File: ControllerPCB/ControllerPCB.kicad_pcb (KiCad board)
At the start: 4 copper layers, 55 x 90 mm, 43 parts, among them J1 USB_B_Micro, J2 A-DF 09 A/KG-T4S, J3 Screw_Terminal_01x02, J4 MotorDriverSocket, J5 UISocket, J6 Pi JST, J7 Conn_02x02_Row_Letter_First, SW1 SW_Push_Dual_x2, SW2 SW_Push_Dual_x2, U1 AMS1117-3.3, U2 ESP32-S3-WROOM-2, U3 LM1084-5.0, U5 TMP236A4DCKR

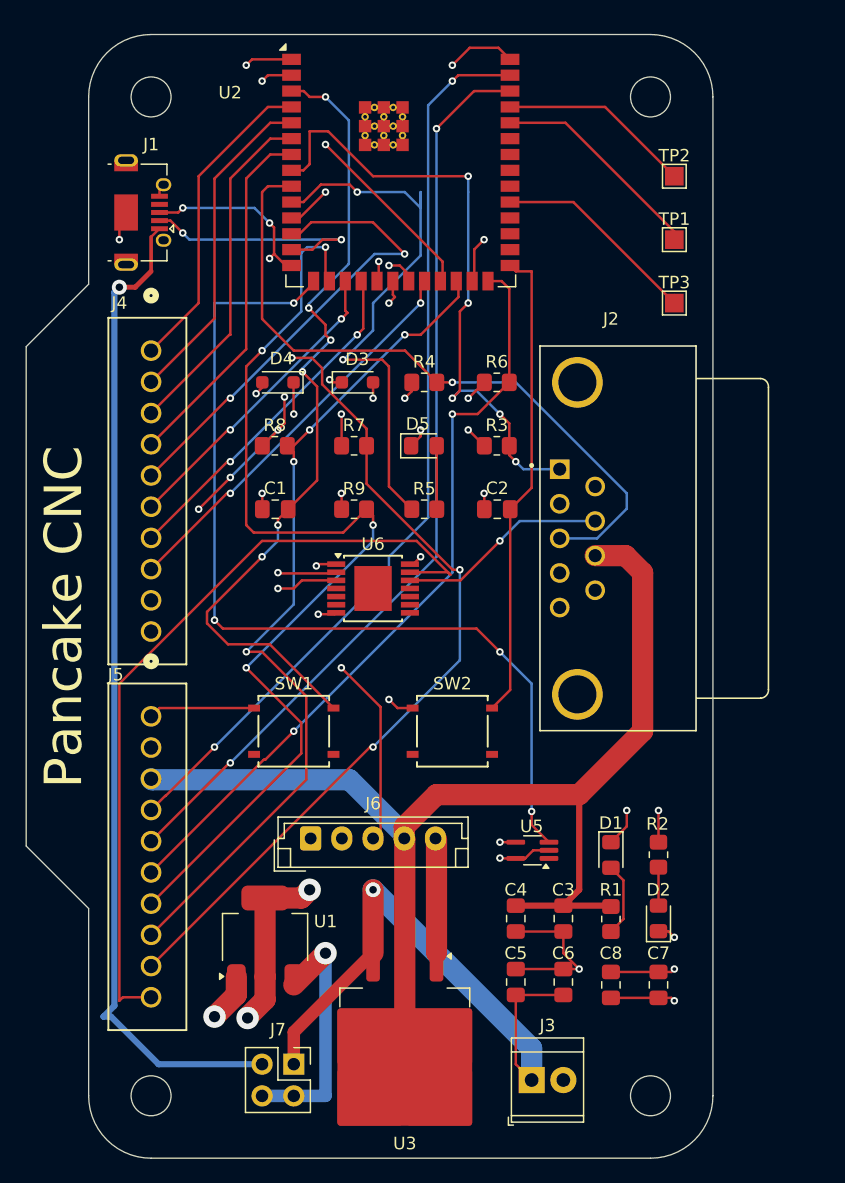
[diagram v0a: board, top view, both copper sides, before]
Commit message: Rev 2 of controller PCB
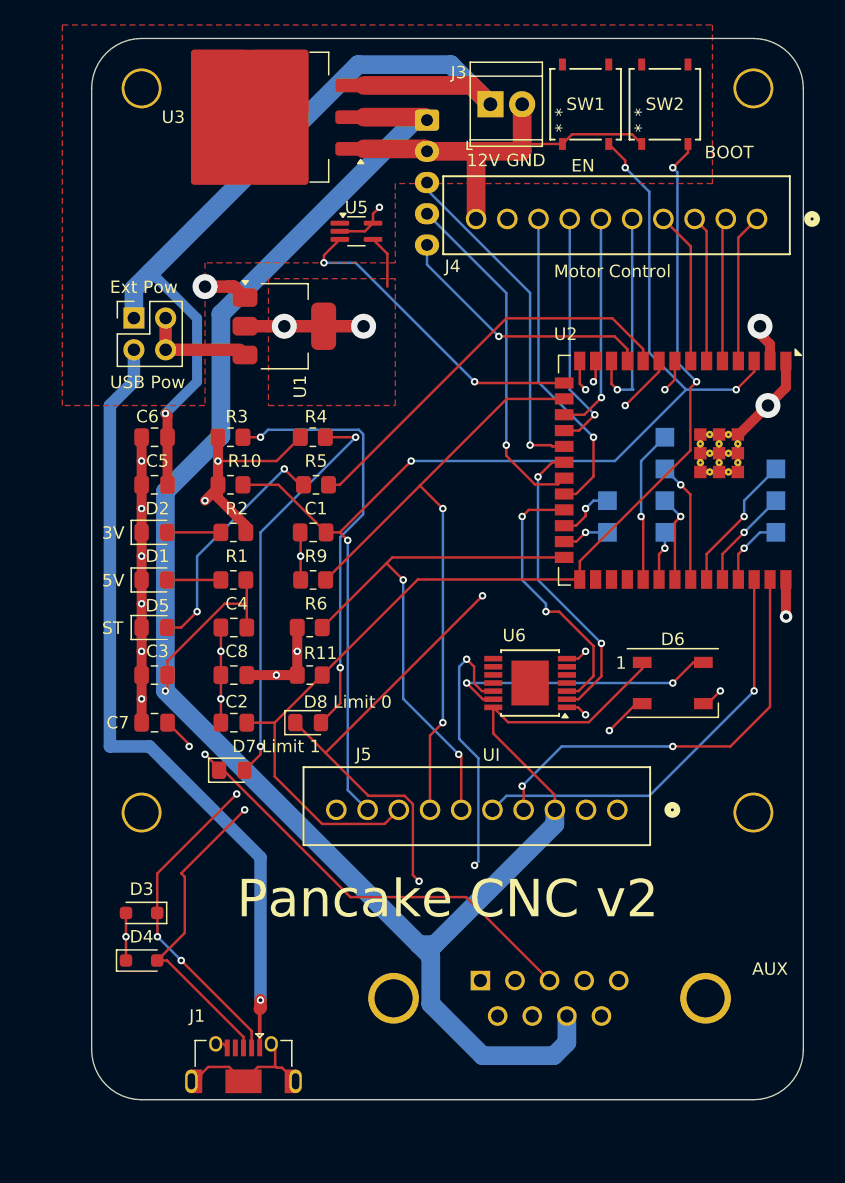
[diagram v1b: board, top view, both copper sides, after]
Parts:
- removed R7, R8: 10k, Resistor_SMD:R_0805_2012Metric_Pad1.20x1.40mm_HandSolder
- added D6: WS2812B, LED_SMD:LED_WS2812B_PLCC4_5.0x5.0mm_P3.2mm, F.Cu at (74.8, 97.9)
- added D7 Limit 1: LED, LED_SMD:LED_0805_2012Metric_Pad1.15x1.40mm_HandSolder, F.Cu at (39.5, 104.9)
- added D8 Limit 0: LED, LED_SMD:LED_0805_2012Metric_Pad1.15x1.40mm_HandSolder, F.Cu at (45.6, 101.1)
- added R10: 10k, Resistor_SMD:R_0805_2012Metric_Pad1.20x1.40mm_HandSolder, F.Cu at (39.4, 82.1)
- added R11: 10k, Resistor_SMD:R_0805_2012Metric_Pad1.20x1.40mm_HandSolder, F.Cu at (45.7, 97.3)
- added TP4: TestPoint, TestPoint:TestPoint_Pad_1.5x1.5mm, B.Cu at (74.2, 85.9)
- added TP5: TestPoint, TestPoint:TestPoint_Pad_1.5x1.5mm, B.Cu at (74.2, 83.3)
- added TP6: TestPoint, TestPoint:TestPoint_Pad_1.5x1.5mm, B.Cu at (74.2, 80.8)
- added TP7: TestPoint, TestPoint:TestPoint_Pad_1.5x1.5mm, B.Cu at (83.0, 80.8)
- added TP8: TestPoint, TestPoint:TestPoint_Pad_1.5x1.5mm, B.Cu at (69.6, 83.3)
- added TP9: TestPoint, TestPoint:TestPoint_Pad_1.5x1.5mm, B.Cu at (69.6, 85.9)
- J2, J6, TP1, TP2, TP3: moved to B.Cu
- R3, R4: value 10k -> 5.1k
- moved J3 78.2 mm to (60.2, 51.6)
- moved U3 75.4 mm to (42.4, 52.6), turned to 180 degrees
- moved J1 70.2 mm to (40.4, 129.8), turned to 0 degrees
- moved J7 61.1 mm to (31.6, 68.7), turned to 90 degrees
- moved J6 58.3 mm to (55.1, 52.9), turned to -90 degrees
- moved SW1 55.4 mm to (67.8, 51.6), turned to 90 degrees
- moved C6 54.5 mm to (33.3, 78.3), turned to 180 degrees
- moved SW2 53.0 mm to (74.2, 51.6), turned to 90 degrees
- moved U5 51.5 mm to (49.4, 61.8), turned to 0 degrees
- moved D2 50.9 mm to (33.3, 85.9), turned to 0 degrees
- moved J4 49.7 mm to (81.5, 60.8), turned to 180 degrees
- moved C5 49.2 mm to (33.3, 82.1), turned to 180 degrees
- moved U1 49.0 mm to (43.7, 69.4), turned to 0 degrees
- moved D4 47.6 mm to (32.2, 120.2), turned to 0 degrees
- moved D3 45.9 mm to (32.2, 116.4), turned to 180 degrees
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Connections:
- C1 pad 2: Net-(SW1A-D) -> Net-(J5-Pin_9)
- C2 pad 2: Net-(SW2A-D) -> Net-(J5-Pin_8)
- J2 pad 1: Net-(U2-IO15) -> Net-(D8-K)
- J2 pad 3: Net-(U2-IO16) -> Net-(D7-K)
- J5 pad 10: Net-(J5-Pin_10) -> Net-(D6-DOUT)
- J6 pad 1: Net-(J6-Pin_1) -> +5V
- J6 pad 2: Net-(J6-Pin_2) -> GND
- J6 pad 4: +5V -> Net-(J6-Pin_4)
- J6 pad 5: GND -> Net-(J6-Pin_5)
- R3 pad 2: Net-(U2-IO15) -> Net-(D8-A)
- R4 pad 2: Net-(U2-IO16) -> Net-(D7-A)
- SW1 pad 2: Net-(SW1A-D) -> (no net)
- SW1 pad 3: (no net) -> Net-(J5-Pin_9)
- SW2 pad 2: Net-(SW2A-D) -> (no net)
- SW2 pad 3: (no net) -> Net-(J5-Pin_8)
- U2 pad 11: Net-(J6-Pin_3) -> Net-(J6-Pin_5)
- U2 pad 19: Net-(J6-Pin_1) -> Net-(J6-Pin_3)
- U2 pad 21: Net-(J6-Pin_2) -> Net-(J6-Pin_4)
- U2 pad 24: Net-(J5-Pin_8) -> Net-(U2-IO47)
- U2 pad 25: Net-(J5-Pin_9) -> Net-(U2-IO48)
- U2 pad 27: Net-(SW2A-D) -> Net-(J5-Pin_8)
- U2 pad 3: Net-(SW1A-D) -> Net-(J5-Pin_9)
- U2 pad 32: unconnected-(U2-MTCK/IO39-Pad32) -> Net-(U2-MTCK/IO39)
- U2 pad 33: unconnected-(U2-MTDO/IO40-Pad33) -> Net-(U2-MTDO/IO40)
- U2 pad 34: unconnected-(U2-MTDI/IO41-Pad34) -> Net-(U2-MTDI/IO41)
- U2 pad 35: unconnected-(U2-MTMS/IO42-Pad35) -> Net-(U2-MTMS/IO42)
- U2 pad 8: Net-(U2-IO15) -> Net-(D8-K)
- U2 pad 9: Net-(U2-IO16) -> Net-(D7-K)
- U6 pad 13: Net-(J5-Pin_10) -> Net-(D6-DIN)
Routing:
- net Net-(D7-K): track 0.00 -> 85.1 mm, vias 0 -> 2
- net Net-(D8-K): track 0.00 -> 71.5 mm, vias 0 -> 3
- net Net-(SW1A-D): track 65.9 -> 0.00 mm, vias 6 -> 0
- net Net-(J5-Pin_10): track 63.7 -> 0.00 mm
- net Net-(U2-IO16): track 56.0 -> 0.00 mm, vias 1 -> 0
- net Net-(J6-Pin_1): track 50.1 -> 0.00 mm, vias 1 -> 0
- net Net-(J6-Pin_2): track 49.8 -> 0.00 mm, vias 1 -> 0
- net Net-(U2-IO15): track 49.7 -> 0.00 mm, vias 5 -> 0
- net Net-(U2-IO3): track 75.0 -> 25.6 mm, vias 4 -> 2
- net Net-(D4-A2): track 26.9 -> 73.0 mm, vias 4 -> 2
- net Net-(D3-A1): track 32.9 -> 73.7 mm, vias 3 -> 4
- net Net-(J5-Pin_5): track 73.7 -> 33.8 mm, vias 2 -> 1
- net Net-(J5-Pin_4): track 73.2 -> 34.6 mm
- net Net-(SW2A-D): track 38.2 -> 0.00 mm
- net Net-(U2-IO21): track 59.1 -> 22.0 mm
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- added copper zone on F.Cu, net +3.3V
- added copper zone on F.Cu, net +5V
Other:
- board size 55 x 90 mm -> 57 x 85 mm
- board text added: "12V"
- board text added: "3V"
- board text added: "5V"
- board text added: "AUX"
- board text added: "BOOT"
- board text added: "EN"
- board text added: "Ext Pow"
- board text added: "GND"
- board text added: "Motor Control"
- board text added: "Pancake CNC v2"
- board text added: "ST"
- board text added: "UI"
- board text added: "USB Pow"
- board text removed: "Pancake CNC"
